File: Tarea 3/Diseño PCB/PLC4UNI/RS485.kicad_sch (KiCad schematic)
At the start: 7 parts, among them U15 RSM3485ECHT_C2992406

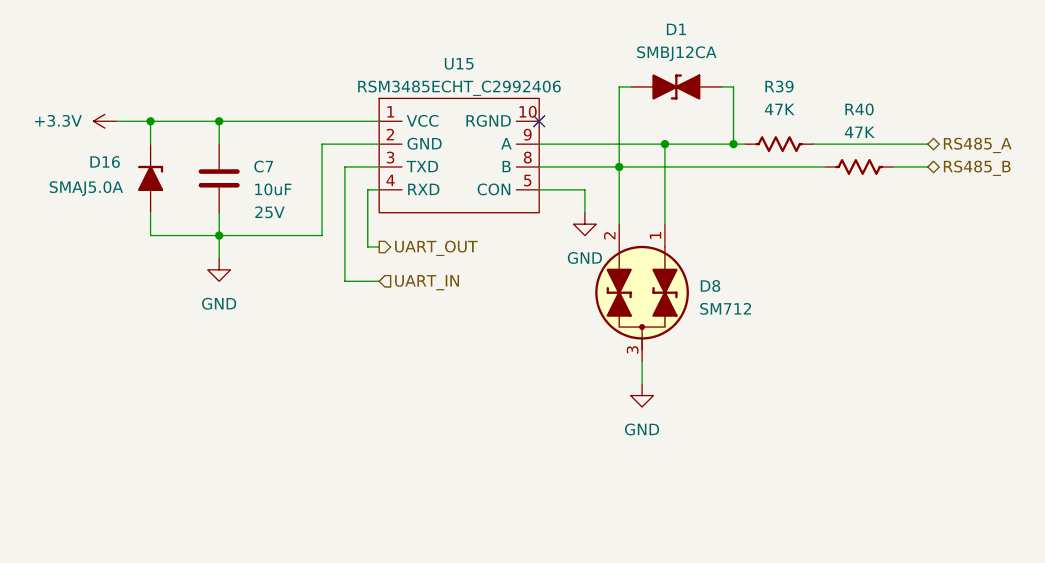
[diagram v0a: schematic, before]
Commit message: tarea 3 - update
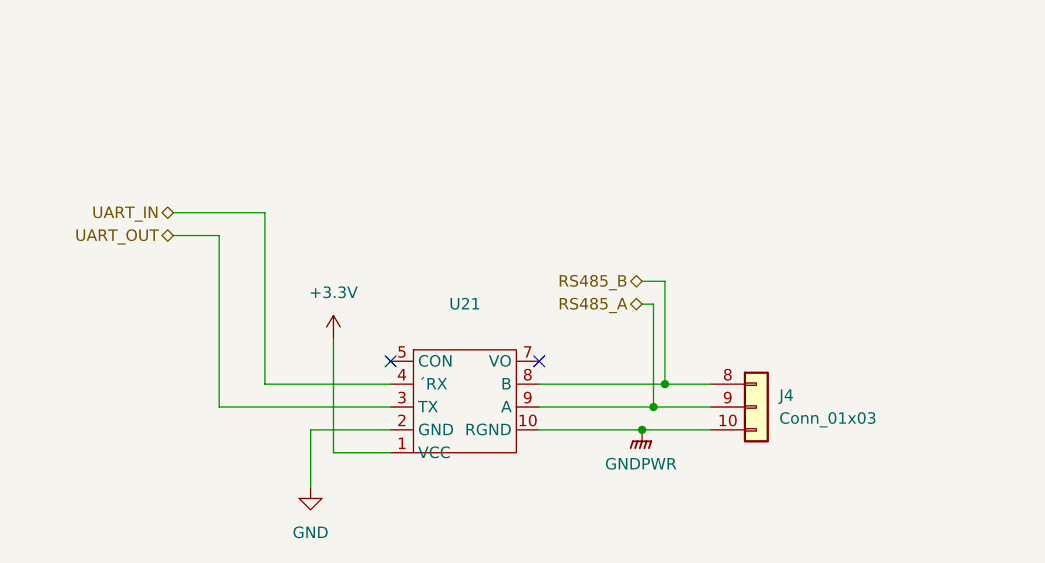
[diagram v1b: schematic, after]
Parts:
- removed C7: 10uF, PCM_Capacitor_SMD_AKL:C_0603_1608Metric, symbol PCM_Capacitor_US_AKL:C_0603
- removed D1: SMBJ12CA, PCM_Diode_SMD_AKL:D_SMB_TVS, symbol PCM_Diode_TVS_AKL:SMBJ12CA
- removed D16: SMAJ5.0A, PCM_Diode_SMD_AKL:D_SMA, symbol PCM_Diode_TVS_AKL:SMAJ5.0A
- removed D8: SM712, PCM_Package_TO_SOT_SMD_AKL:SOT-23, symbol PCM_Diode_TVS_AKL:SM712
- removed R39, R40: 47K, PCM_Resistor_SMD_AKL:R_0603_1608Metric, symbol PCM_Resistor_US_AKL:R_0603
- removed U15: RSM3485ECHT_C2992406, Biblioteca_BryanFernandez_Huellas:YLPTEC RSM3485ECHT, symbol New_Library:RSM3485ECHT_C2992406
- added J4: Conn_01x03, Connector_PinHeader_2.54mm:PinHeader_1x03_P2.54mm_Vertical, symbol RS_MOD_PRO:Conn_01x03
- added U21: ~, rs485_footprint:SOIC127P600X175-8N, symbol RS485ULTRA:ULTRADONE
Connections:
- net +3.3V: now also U21.1 (VCC)
- net GND: now also U21.2 (GND)
- net RS485_A: now also J4.9 (Pin_2), U21.9 (A)
- net RS485_B: now also J4.8 (Pin_1), U21.8 (B)
- net UART_IN: now also U21.4 (´RX)
- net UART_OUT: now also U21.3 (TX)
- new net GNDPWR: J4.10 (Pin_3), U21.10 (RGND)
- no-connect marks 1 -> 2
